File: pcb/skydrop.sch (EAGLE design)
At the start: 107 parts, among them IC1 RT9193-33GB, IC2 MCP73831/OT, IC3 STM809SWX6F, IC4 MS5611-01BA03, IC5 MCP23S17SO, Q1 BSS84, Q10 BSS84, Q2 BSS123, Q3 BSS123, Q4 BSS123, Q5 BSS84, Q6 BSS84, Q7 BSS123, Q8 BSS84, Q9 BSS84, SW1 431256083736, U2 W25Q16BVSS

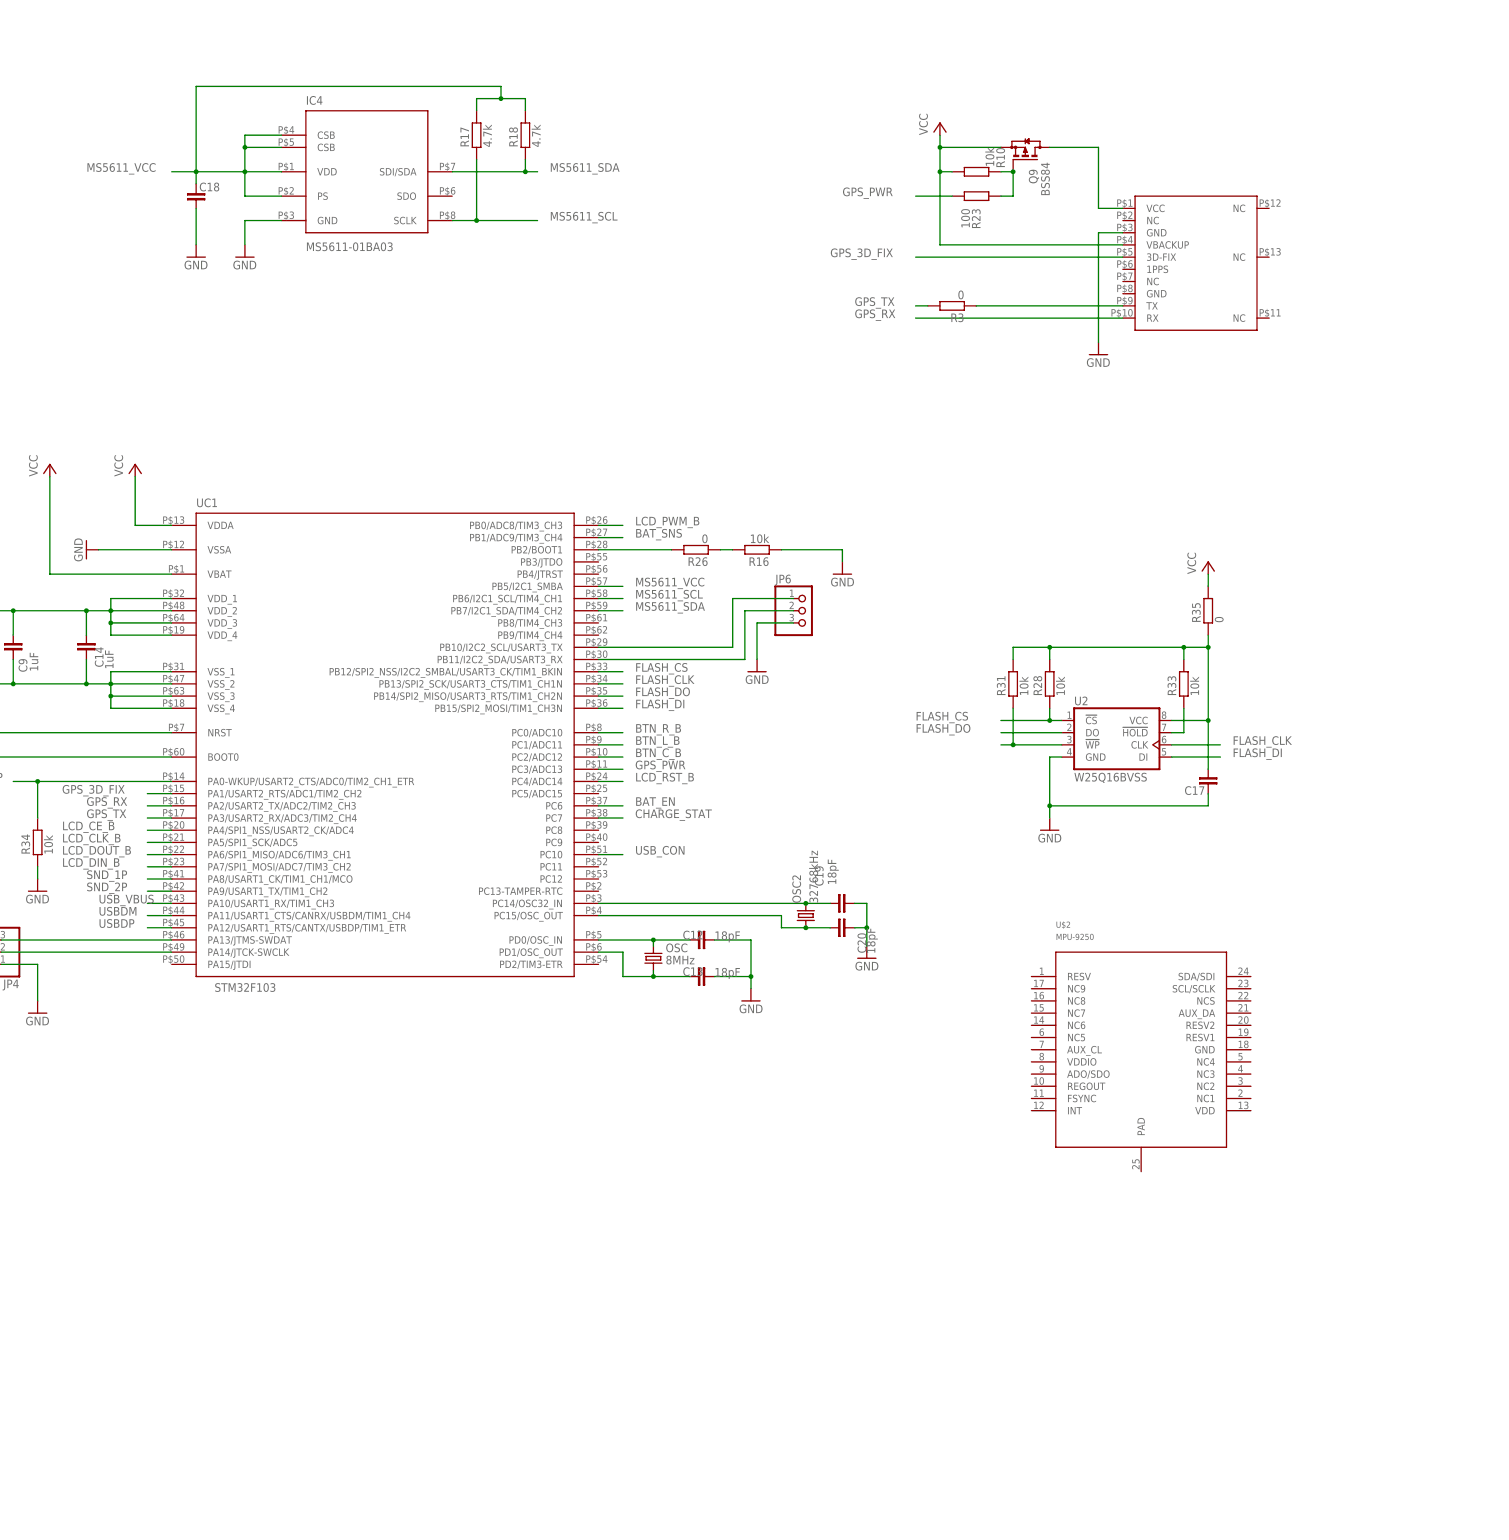
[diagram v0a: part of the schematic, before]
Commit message: [pcb] improve
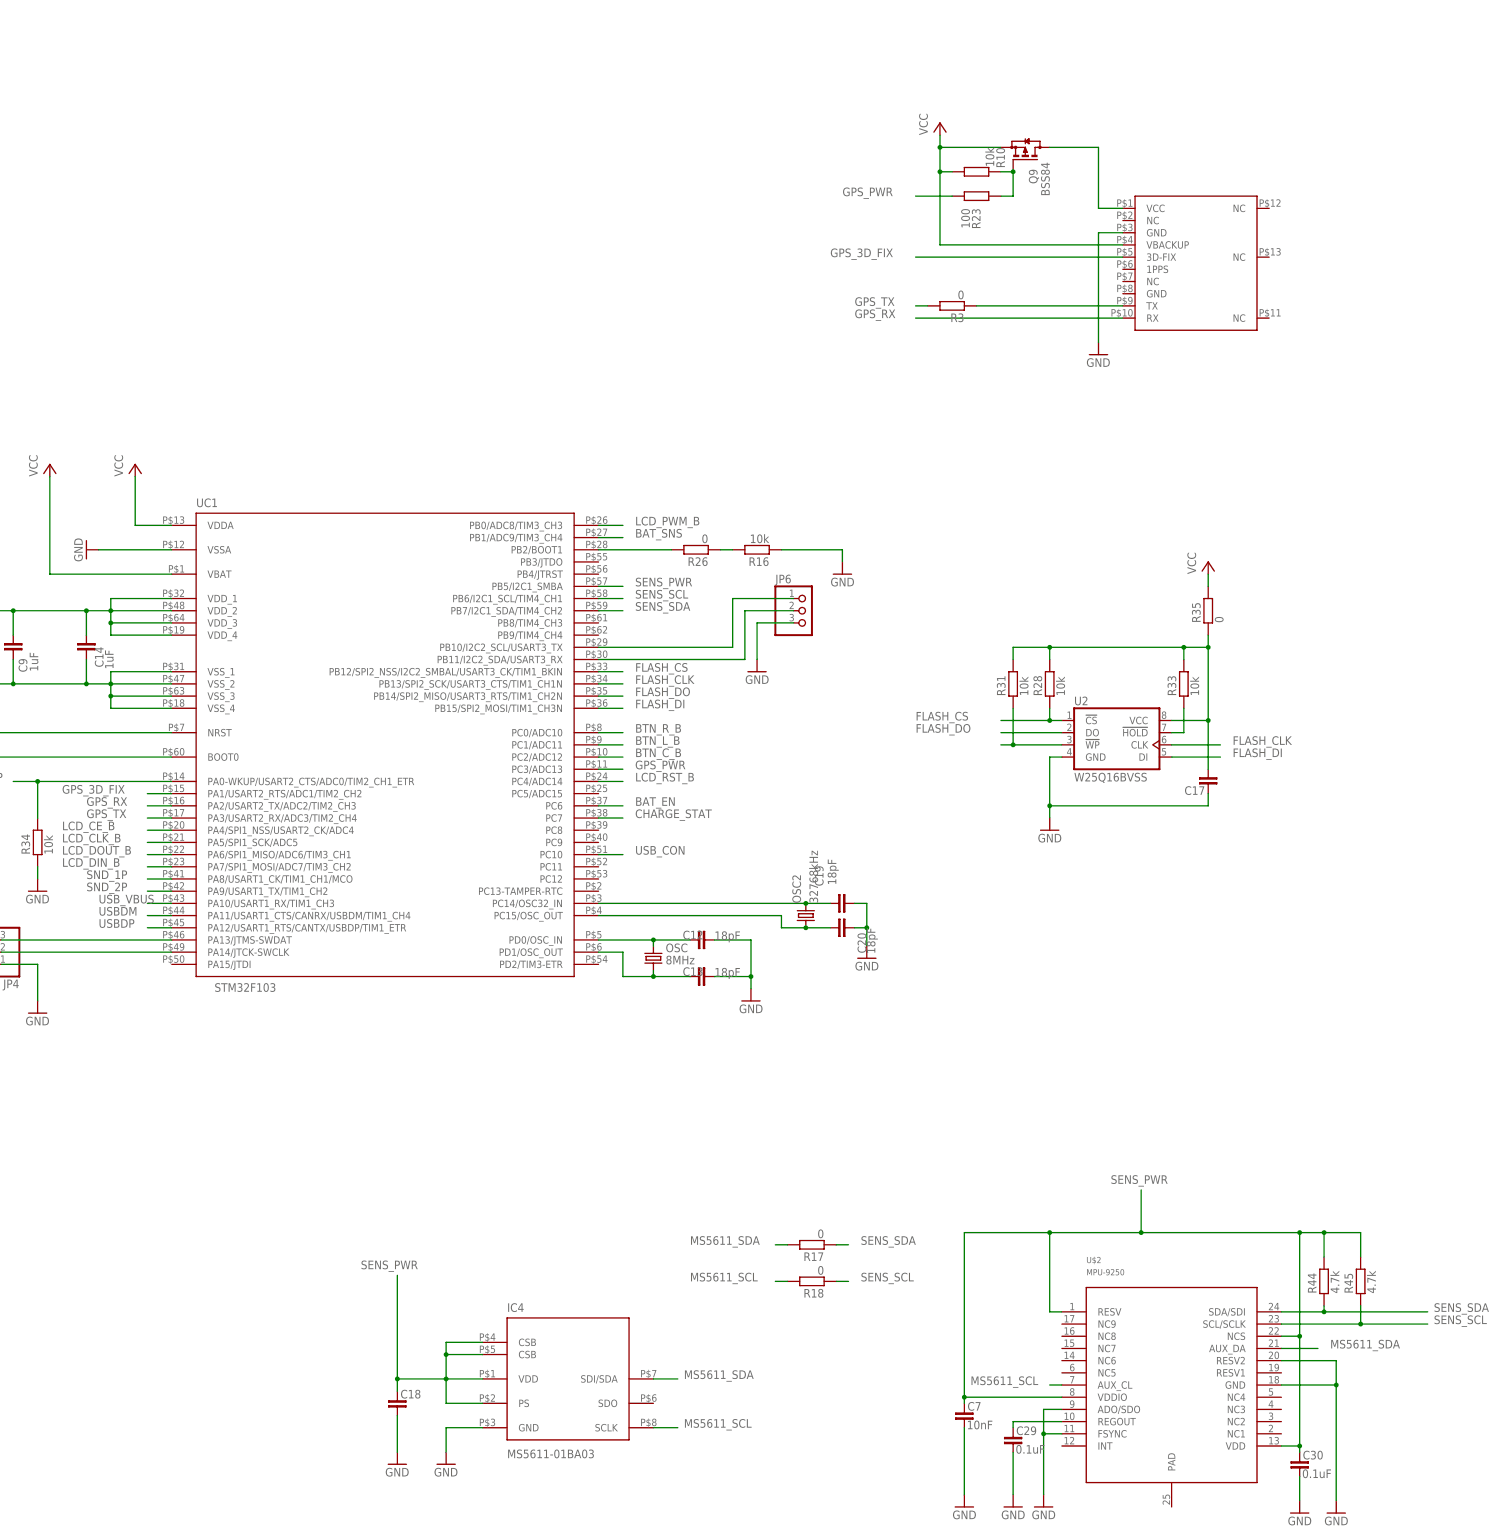
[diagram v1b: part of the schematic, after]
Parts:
- added C29, C30: 0.1uF, skydrop:C_0805
- added C7: 10nF, skydrop:C_0805
- added R44, R45: 4.7k, skydrop:R_0805
- R17, R18: value 4.7k -> 0; device skydrop:R_0805 -> skydrop:R_1206
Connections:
- removed net MS5611_VCC: C18.1, IC4.CSB@1, IC4.CSB@2, IC4.PS, IC4.VDD, R17.2, R18.2, UC1.PB5/I2C1_SMBA
- new net N$66: C29.1, U$2.REGOUT
- new net SENS_PWR: C18.1, C30.1, C7.1, IC4.CSB@1, IC4.CSB@2, IC4.PS, IC4.VDD, R44.2, R45.2, U$2.NCS, U$2.RESV, U$2.VDD, U$2.VDDIO, UC1.PB5/I2C1_SMBA
- new net SENS_SCL: R18.1, R45.1, U$2.SCL/SCLK, UC1.PB6/I2C1_SCL/TIM4_CH1
- new net SENS_SDA: R17.1, R44.1, U$2.SDA/SDI, UC1.PB7/I2C1_SDA/TIM4_CH2
- net GND: now also C29.2, C30.2, C7.2, U$2.ADO/SDO, U$2.FSYNC, U$2.GND, U$2.RESV2
- net MS5611_SCL: now also R18.2, U$2.AUX_CL; no longer R17.1, UC1.PB6/I2C1_SCL/TIM4_CH1
- net MS5611_SDA: now also R17.2, U$2.AUX_DA; no longer R18.1, UC1.PB7/I2C1_SDA/TIM4_CH2
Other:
- moved on the sheet: C18, IC4, R17, R18, U$2
